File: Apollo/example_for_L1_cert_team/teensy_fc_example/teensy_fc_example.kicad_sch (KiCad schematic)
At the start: 4 parts, among them U1 BMP390

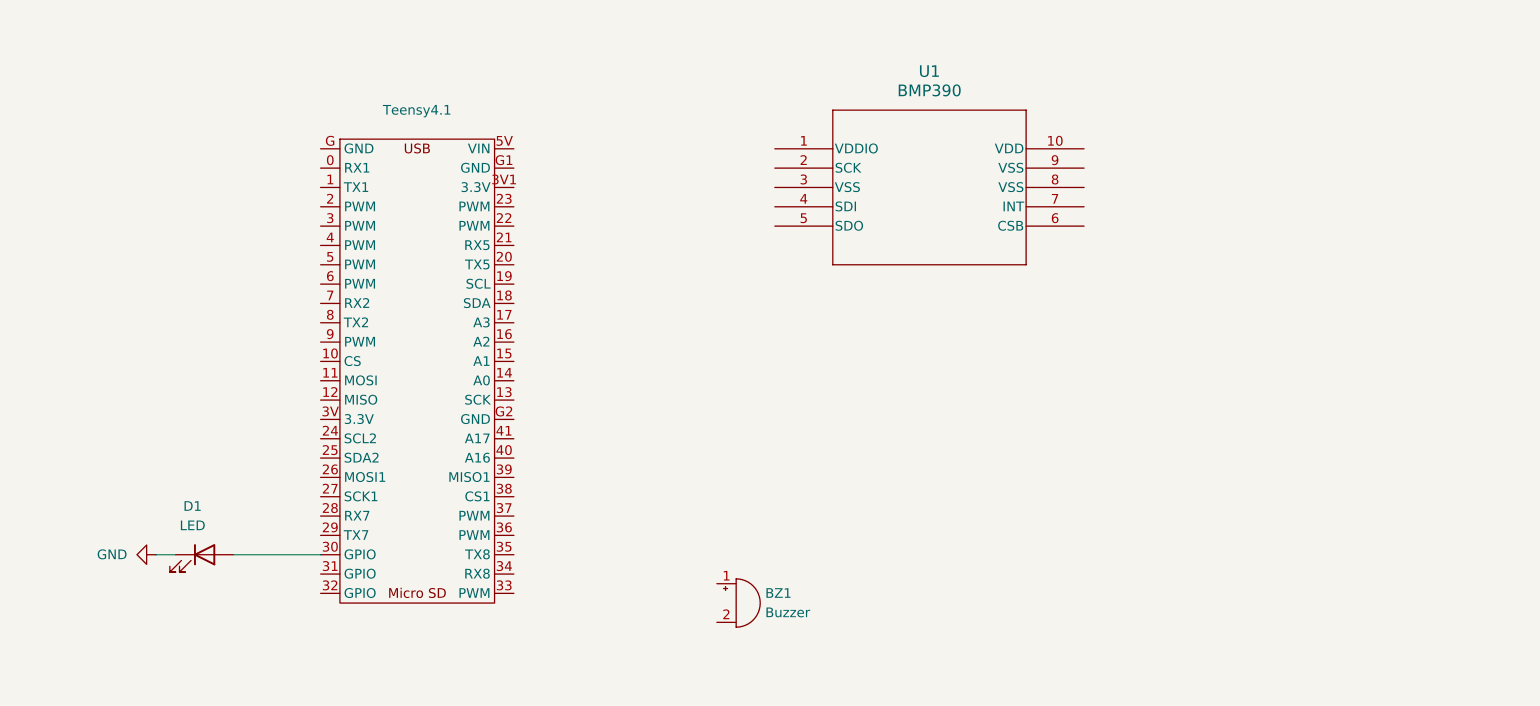
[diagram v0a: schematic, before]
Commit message: Push
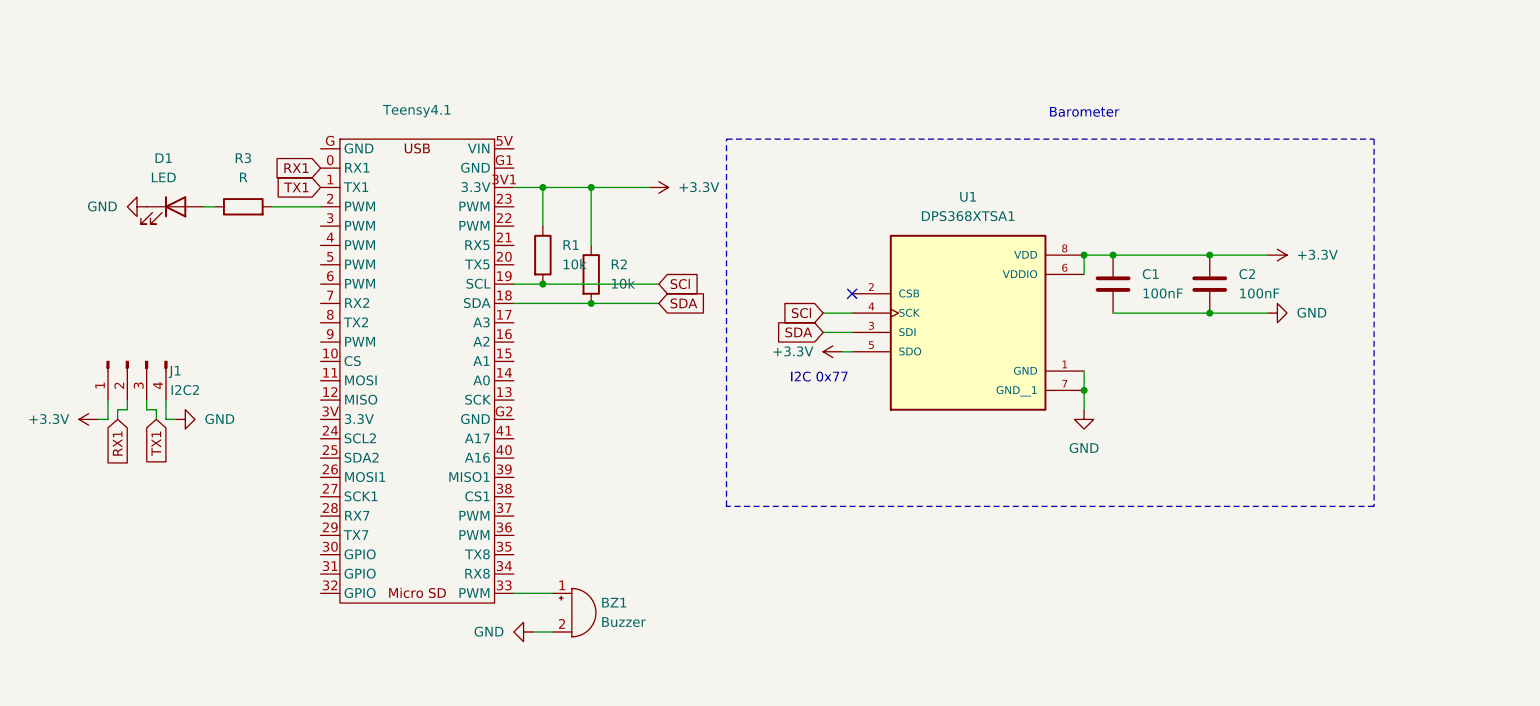
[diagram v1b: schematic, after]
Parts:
- removed U1: BMP390, 10LGA_2X2X0p75_BOS, symbol my_library:BMP390
- added C1, C2: 100nF, symbol Device:C
- added J1: I2C2, Connector_PinHeader_2.54mm:PinHeader_1x04_P2.54mm_Vertical, symbol Connector:Conn_01x04_Pin
- added R1, R2: 10k, symbol Device:R
- added R3: R, symbol Device:R
- added U1: DPS368XTSA1, DPS368XTSA1:XDCR_DPS368XTSA1, symbol my_library:DPS368XTSA1
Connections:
- net GND: now also BZ1.2 (-), C1.2, C2.2, J1.4 (Pin_4), U1.1 (GND), U1.7 (GND__1)
- net at D1.2 (A): now also R3.1; no longer Teensy4.1.30 (GPIO)
- net at BZ1.1 (+): now also Teensy4.1.33 (PWM)
- net RX1: now reaches Teensy4.1.0 (RX1)
- net RX1: now also J1.2 (Pin_2)
- net TX1: now reaches Teensy4.1.1 (TX1)
- net TX1: now also J1.3 (Pin_3)
- net SDA: now reaches Teensy4.1.18 (SDA)
- net SDA: now also R2.2, U1.3 (SDI)
- net SCl: now reaches Teensy4.1.19 (SCL)
- net SCl: now also R1.2, U1.4 (SCK)
- net at Teensy4.1.2 (PWM): now also R3.2
- net +3.3V: now reaches Teensy4.1.3V1 (3.3V)
- net +3.3V: now also C1.1, C2.1, J1.1 (Pin_1), R1.1, R2.1, U1.5 (SDO), U1.6 (VDDIO), U1.8 (VDD)
- no-connect marks 0 -> 1
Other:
- note added: "Barometer"
- note added: "I2C 0x77"
- moved on the sheet: BZ1, D1

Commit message: louie example
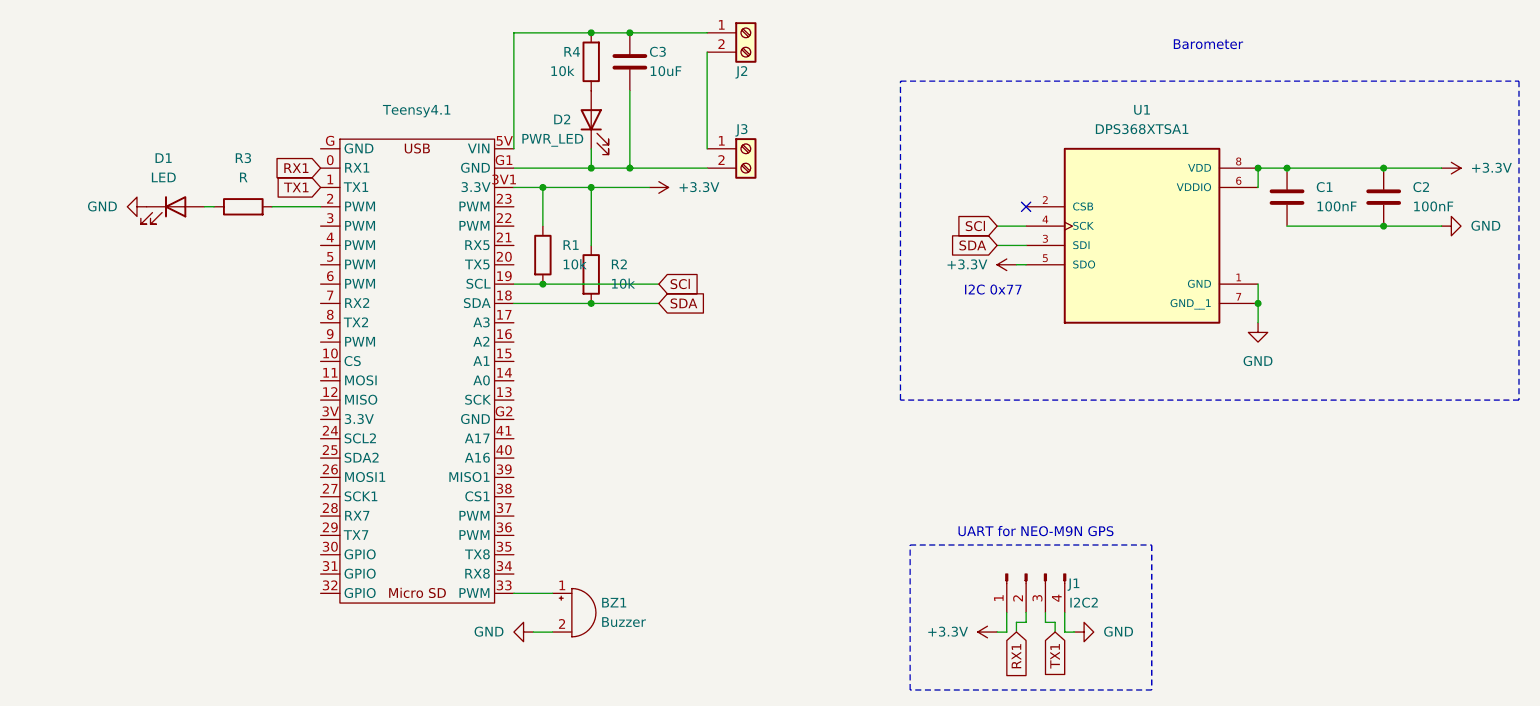
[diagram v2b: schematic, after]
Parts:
- added C3: 10uF, Capacitor_SMD:C_0805_2012Metric, symbol Device:C
- added D2: PWR_LED, LED_SMD:LED_0805_2012Metric_Pad1.15x1.40mm_HandSolder, symbol Device:LED
- added J2, J3: Screw_Terminal_01x02, TerminalBlock_4Ucon:TerminalBlock_4Ucon_1x02_P3.50mm_Vertical, symbol Connector:Screw_Terminal_01x02
- added R4: 10k, Resistor_SMD:R_0805_2012Metric, symbol Device:R
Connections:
- net at Teensy4.1.5V (VIN): now also C3.1, J2.1 (Pin_1), R4.2
- net at Teensy4.1.G1 (GND): now also C3.2, D2.1 (K), J3.2 (Pin_2)
- new net: J2.2 (Pin_2), J3.1 (Pin_1)
- new net: D2.2 (A), R4.1
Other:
- note added: "UART for NEO-M9N GPS"
- moved on the sheet: C1, C2, J1, U1
